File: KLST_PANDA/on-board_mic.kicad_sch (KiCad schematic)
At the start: 0 parts

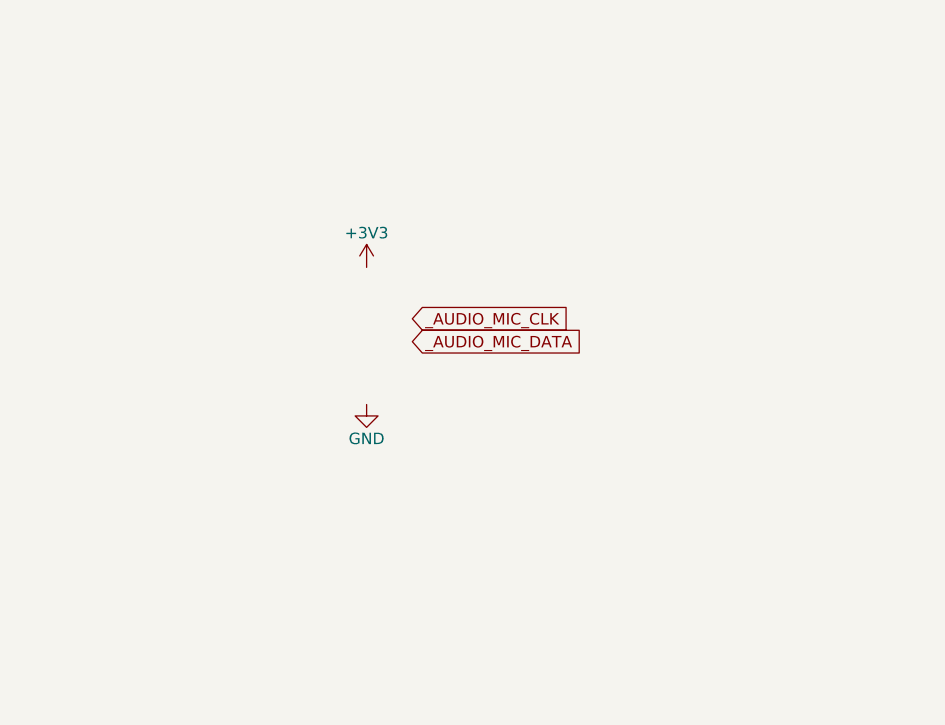
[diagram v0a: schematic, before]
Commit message: added MEMS mics
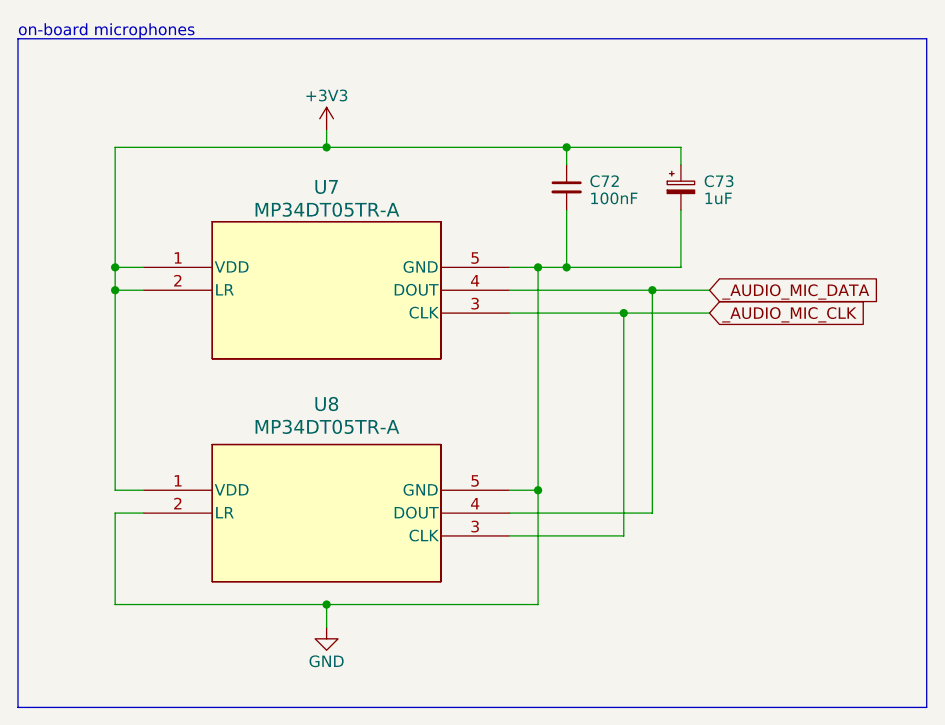
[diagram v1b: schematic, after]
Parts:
- added C72: 100nF, symbol Device:C_Small
- added C73: 1uF, symbol Device:C_Polarized_Small
- added U7, U8: MP34DT05TR-A, MP34DT05TR-A_STM, symbol MP34DT05TR-A:MP34DT05TR-A
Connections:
- net +3V3: now also C72.1, C73.1, U7.1 (VDD), U7.2 (LR), U8.1 (VDD)
- net GND: now also C72.2, C73.2, U7.5 (GND), U8.2 (LR), U8.5 (GND)
- net _AUDIO_MIC_CLK: now also U7.3 (CLK), U8.3 (CLK)
- net _AUDIO_MIC_DATA: now also U7.4 (DOUT), U8.4 (DOUT)
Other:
- note added: "on-board microphones"
